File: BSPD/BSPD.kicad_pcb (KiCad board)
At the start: 2 copper layers, 1 part, among them J1 Conn_01x08

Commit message: finished V1 of bspd
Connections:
- J1 pad 1: unconnected-(J1-Pin_1-Pad1) -> +5V
- J1 pad 2: unconnected-(J1-Pin_2-Pad2) -> GND
- J1 pad 3: unconnected-(J1-Pin_3-Pad3) -> /Rear_Brake_Sensor
- J1 pad 4: unconnected-(J1-Pin_4-Pad4) -> /Front_Brake_Sensor
- J1 pad 5: unconnected-(J1-Pin_5-Pad5) -> /Current_Sensor_Output
- J1 pad 6: unconnected-(J1-Pin_6-Pad6) -> /Current_Sensor_VREF
- J1 pad 7: unconnected-(J1-Pin_7-Pad7) -> /Fault
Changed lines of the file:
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@@
 	)
 	(net 0 "")
-	(net 1 "unconnected-(J1-Pin_6-Pad6)")
+	(net 1 "/Current_Sensor_Output")
 	(net 2 "unconnected-(J1-Pin_8-Pad8)")
-	(net 3 "unconnected-(J1-Pin_3-Pad3)")
-	(net 4 "unconnected-(J1-Pin_4-Pad4)")
-	(net 5 "unconnected-(J1-Pin_7-Pad7)")
-	(net 6 "unconnected-(J1-Pin_2-Pad2)")
-	(net 7 "unconnected-(J1-Pin_1-Pad1)")
-	(net 8 "unconnected-(J1-Pin_5-Pad5)")
+	(net 3 "GND")
+	(net 4 "/Front_Brake_Sensor")
+	(net 5 "/Rear_Brake_Sensor")
+	(net 6 "+5V")
+	(net 7 "/Current_Sensor_VREF")
+	(net 8 "/Fault")
 	(footprint "Connector_Molex:Molex_Nano-Fit_105313-xx08_1x08_P2.50mm_Horizontal"
 		(layer "F.Cu")
@@
 			(remove_unused_layers no)
 			(roundrect_rratio 0.147059)
-			(net 7 "unconnected-(J1-Pin_1-Pad1)")
+			(net 6 "+5V")
 			(pinfunction "Pin_1")
 			(pintype "passive")
@@
 			(layers "*.Cu" "*.Mask")
 			(remove_unused_layers no)
-			(net 6 "unconnected-(J1-Pin_2-Pad2)")
+			(net 3 "GND")
 			(pinfunction "Pin_2")
 			(pintype "passive")
@@
 			(layers "*.Cu" "*.Mask")
 			(remove_unused_layers no)
-			(net 3 "unconnected-(J1-Pin_3-Pad3)")
+			(net 5 "/Rear_Brake_Sensor")
 			(pinfunction "Pin_3")
 			(pintype "passive")
@@
 			(layers "*.Cu" "*.Mask")
 			(remove_unused_layers no)
-			(net 4 "unconnected-(J1-Pin_4-Pad4)")
+			(net 4 "/Front_Brake_Sensor")
 			(pinfunction "Pin_4")
 			(pintype "passive")
@@
 			(layers "*.Cu" "*.Mask")
 			(remove_unused_layers no)
-			(net 8 "unconnected-(J1-Pin_5-Pad5)")
+			(net 1 "/Current_Sensor_Output")
 			(pinfunction "Pin_5")
 			(pintype "passive")
@@
 			(layers "*.Cu" "*.Mask")
 			(remove_unused_layers no)
-			(net 1 "unconnected-(J1-Pin_6-Pad6)")
+			(net 7 "/Current_Sensor_VREF")
 			(pinfunction "Pin_6")
 			(pintype "passive")
@@
 			(layers "*.Cu" "*.Mask")
 			(remove_unused_layers no)
-			(net 5 "unconnected-(J1-Pin_7-Pad7)")
+			(net 8 "/Fault")
 			(pinfunction "Pin_7")
 			(pintype "passive")

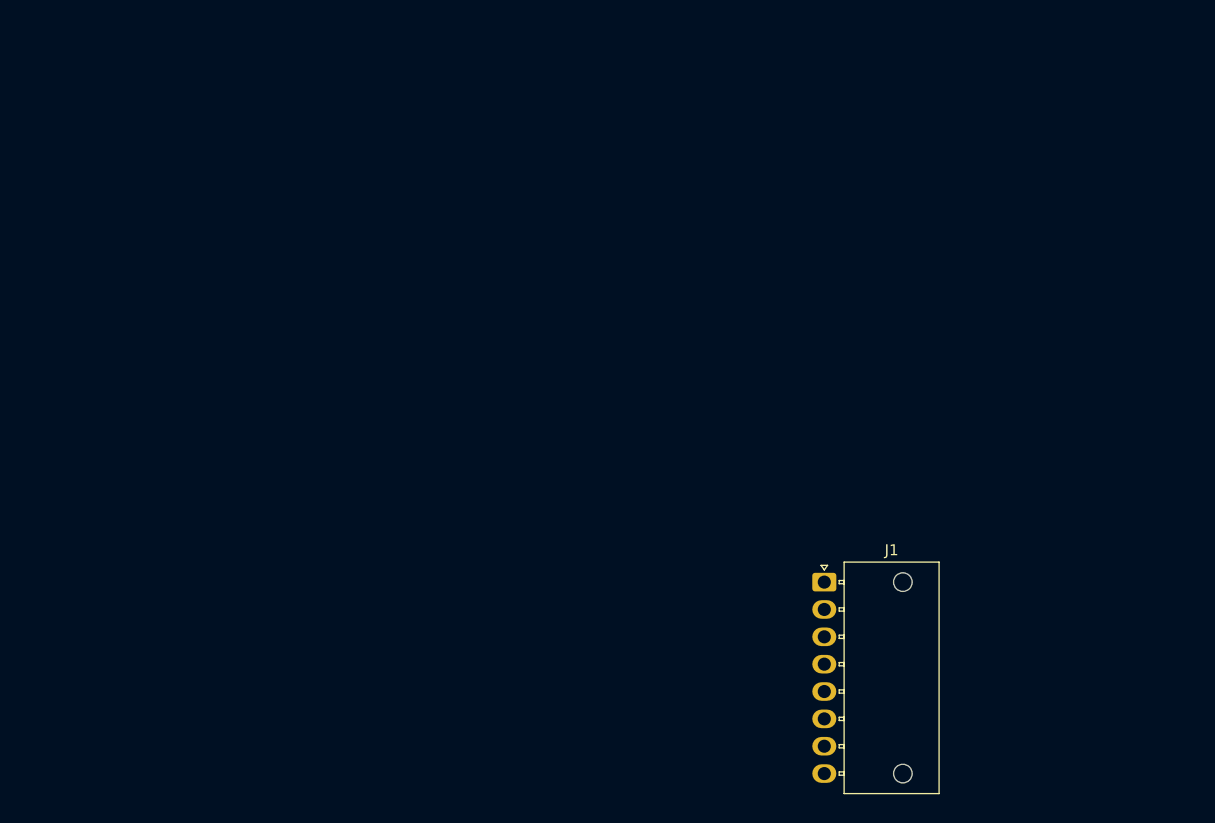
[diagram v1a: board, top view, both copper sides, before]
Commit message: Finished BSPD
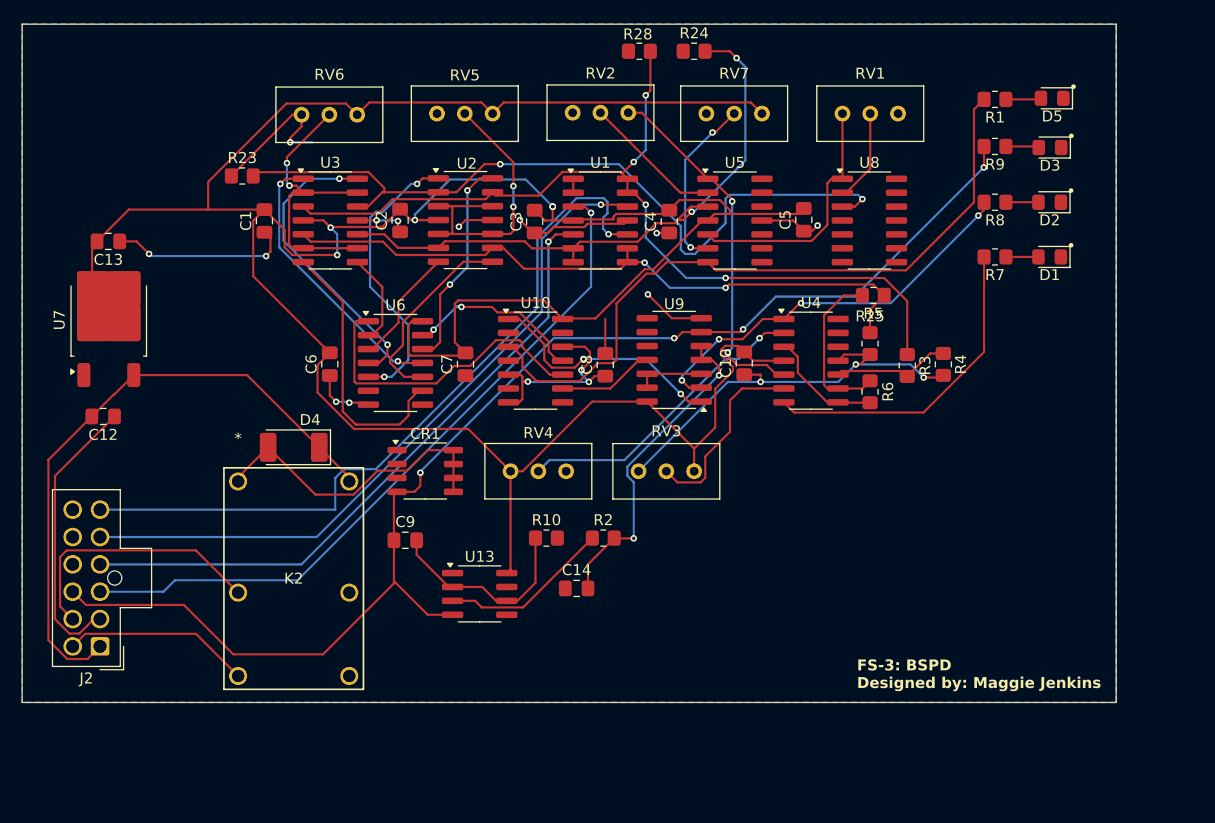
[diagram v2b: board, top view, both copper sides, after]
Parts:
- removed J1: Conn_01x08, Connector_Molex:Molex_Nano-Fit_105313-xx08_1x08_P2.50mm_Horizontal
- added C1: 0.1μF, Capacitor_SMD:C_0805_2012Metric_Pad1.18x1.45mm_HandSolder, F.Cu at (35.1, 33.0)
- added C10: 0.1μF, Capacitor_SMD:C_0805_2012Metric_Pad1.18x1.45mm_HandSolder, F.Cu at (79.0, 46.0)
- added C12: 0.33µF, Capacitor_SMD:C_0805_2012Metric_Pad1.18x1.45mm_HandSolder, F.Cu at (20.4, 50.9)
- added C13: 0.1µF, Capacitor_SMD:C_0805_2012Metric_Pad1.18x1.45mm_HandSolder, F.Cu at (20.9, 34.9)
- added C14: 0.1μF, Capacitor_SMD:C_0805_2012Metric_Pad1.18x1.45mm_HandSolder, F.Cu at (63.7, 66.6)
- added C2: 0.1μF, Capacitor_SMD:C_0805_2012Metric_Pad1.18x1.45mm_HandSolder, F.Cu at (47.5, 32.9)
- added C3: 0.1μF, Capacitor_SMD:C_0805_2012Metric_Pad1.18x1.45mm_HandSolder, F.Cu at (59.8, 33.0)
- added C4: 0.1μF, Capacitor_SMD:C_0805_2012Metric_Pad1.18x1.45mm_HandSolder, F.Cu at (72.1, 33.0)
- added C5: 0.1μF, Capacitor_SMD:C_0805_2012Metric_Pad1.18x1.45mm_HandSolder, F.Cu at (84.4, 32.9)
- added C6: 0.1μF, Capacitor_SMD:C_0805_2012Metric_Pad1.18x1.45mm_HandSolder, F.Cu at (41.1, 46.1)
- added C7: 0.1μF, Capacitor_SMD:C_0805_2012Metric_Pad1.18x1.45mm_HandSolder, F.Cu at (53.5, 46.1)
- added C8: 0.1μF, Capacitor_SMD:C_0805_2012Metric_Pad1.18x1.45mm_HandSolder, F.Cu at (66.3, 46.1)
- added C9: 1µF, Capacitor_SMD:C_0805_2012Metric_Pad1.18x1.45mm_HandSolder, F.Cu at (48.0, 62.2)
- added CR1: STS6NF20V, Package_SO:SO-8_3.9x4.9mm_P1.27mm, F.Cu at (49.8, 55.8)
- added D1: QBLP631-R3A, FS_3_Global_Footprint_Library:LED_0805_2012Metric_Pad1.15x1.40mm_HandSolder_CathodeDot, F.Cu at (106.9, 36.3)
- added D2: QBLP631-R3A, FS_3_Global_Footprint_Library:LED_0805_2012Metric_Pad1.15x1.40mm_HandSolder_CathodeDot, F.Cu at (106.9, 31.3)
- added D3: QBLP631-R3A, FS_3_Global_Footprint_Library:LED_0805_2012Metric_Pad1.15x1.40mm_HandSolder_CathodeDot, F.Cu at (106.9, 26.3)
- added D4: D, Diode_SMD:D_2010_5025Metric_Pad1.52x2.65mm_HandSolder, F.Cu at (37.8, 53.7)
- added D5: QBLP631-R3A, FS_3_Global_Footprint_Library:LED_0805_2012Metric_Pad1.15x1.40mm_HandSolder_CathodeDot, F.Cu at (107.1, 21.8)
- added J2: Conn_01x12, Connector_Molex:Molex_Nano-Fit_105310-xx12_2x06_P2.50mm_Vertical, F.Cu at (20.1, 71.9)
- added K2: DK1A1B-12V, FS_3_Global_Footprint_Library:DK1A1B, F.Cu at (32.7, 56.8)
- added R1: 300, Resistor_SMD:R_0805_2012Metric_Pad1.20x1.40mm_HandSolder, F.Cu at (101.9, 21.9)
- added R10: 430k, Resistor_SMD:R_0805_2012Metric_Pad1.20x1.40mm_HandSolder, F.Cu at (60.9, 62.0)
- added R2: 10k, Resistor_SMD:R_0805_2012Metric_Pad1.20x1.40mm_HandSolder, F.Cu at (66.1, 62.0)
- added R23: 100k, Resistor_SMD:R_0805_2012Metric_Pad1.20x1.40mm_HandSolder, F.Cu at (33.1, 28.9)
- added R24: 100k, Resistor_SMD:R_0805_2012Metric_Pad1.20x1.40mm_HandSolder, F.Cu at (74.4, 17.5)
- added R25: 100k, Resistor_SMD:R_0805_2012Metric_Pad1.20x1.40mm_HandSolder, F.Cu at (90.5, 44.2)
- added R28: 100k, Resistor_SMD:R_0805_2012Metric_Pad1.20x1.40mm_HandSolder, F.Cu at (69.4, 17.5)
- added R3: 1k, Resistor_SMD:R_0805_2012Metric_Pad1.20x1.40mm_HandSolder, F.Cu at (93.9, 46.2)
- added R4: 20k, Resistor_SMD:R_0805_2012Metric_Pad1.20x1.40mm_HandSolder, F.Cu at (97.2, 46.1)
- added R5: 1k, Resistor_SMD:R_0805_2012Metric_Pad1.20x1.40mm_HandSolder, F.Cu at (90.8, 39.8)
- added R6: 20k, Resistor_SMD:R_0805_2012Metric_Pad1.20x1.40mm_HandSolder, F.Cu at (90.5, 48.6)
- added R7: 300, Resistor_SMD:R_0805_2012Metric_Pad1.20x1.40mm_HandSolder, F.Cu at (101.9, 36.3)
- added R8: 300, Resistor_SMD:R_0805_2012Metric_Pad1.20x1.40mm_HandSolder, F.Cu at (101.9, 31.3)
- added R9: 300, Resistor_SMD:R_0805_2012Metric_Pad1.20x1.40mm_HandSolder, F.Cu at (101.9, 26.2)
- added RV1: 3296W_10K, Potentiometer_THT:Potentiometer_Bourns_3296W_Vertical, F.Cu at (93.1, 23.2)
- added RV2: 3296W_10K, Potentiometer_THT:Potentiometer_Bourns_3296W_Vertical, F.Cu at (63.3, 23.1)
- added RV3: 3296W_10K, Potentiometer_THT:Potentiometer_Bourns_3296W_Vertical, F.Cu at (74.4, 55.9)
- added RV4: 3296W_10K, Potentiometer_THT:Potentiometer_Bourns_3296W_Vertical, F.Cu at (57.6, 55.9)
- added RV5: 3296W_10K, Potentiometer_THT:Potentiometer_Bourns_3296W_Vertical, F.Cu at (56.0, 23.2)
- added RV6: 3296W_10K, Potentiometer_THT:Potentiometer_Bourns_3296W_Vertical, F.Cu at (43.6, 23.3)
- added RV7: 3296W_10K, Potentiometer_THT:Potentiometer_Bourns_3296W_Vertical, F.Cu at (80.6, 23.2)
- added U1: MCP6004, Package_SO:SOIC-14_3.9x8.7mm_P1.27mm, F.Cu at (65.8, 32.9)
- added U10: 4072, Package_SO:SOIC-14_3.9x8.7mm_P1.27mm, F.Cu at (59.9, 45.8)
- added U13: LM555xM, Package_SO:SOIC-8_3.9x4.9mm_P1.27mm, F.Cu at (54.8, 67.1)
- added U2: MCP6004, Package_SO:SOIC-14_3.9x8.7mm_P1.27mm, F.Cu at (53.5, 32.9)
- added U3: MCP6004, Package_SO:SOIC-14_3.9x8.7mm_P1.27mm, F.Cu at (41.2, 32.9)
- added U4: MCP6004, Package_SO:SOIC-14_3.9x8.7mm_P1.27mm, F.Cu at (85.1, 45.8)
- added U5: MCP6004, Package_SO:SOIC-14_3.9x8.7mm_P1.27mm, F.Cu at (78.1, 32.9)
- added U6: 4072, Package_SO:SOIC-14_3.9x8.7mm_P1.27mm, F.Cu at (47.1, 46.0)
- added U7: LD1086DT50TR, Package_TO_SOT_SMD:TO-252-2, F.Cu at (20.9, 42.0)
- added U8: MCP6004, Package_SO:SOIC-14_3.9x8.7mm_P1.27mm, F.Cu at (90.4, 32.9)
- added U9: 74HC00, Package_SO:SOIC-14_3.9x8.7mm_P1.27mm, F.Cu at (72.6, 45.7)
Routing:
- net +5V: track 0.00 -> 290.0 mm, vias 0 -> 5
- net GND: track 0.00 -> 151.6 mm, vias 0 -> 18
- net /BSPD_Fault_LOW: track 0.00 -> 118.1 mm, vias 0 -> 4
- net /Current_Sensor_Output_Buffered: track 0.00 -> 81.9 mm, vias 0 -> 4
- net /Rear_Brake_Buffered: track 0.00 -> 71.7 mm, vias 0 -> 2
- net /Current_Sensor_VREF: track 0.00 -> 68.8 mm, vias 0 -> 1
- net /Rear_Brake_Sensor: track 0.00 -> 65.0 mm, vias 0 -> 1
- net /Current_Sensor_Output: track 0.00 -> 64.8 mm, vias 0 -> 1
- net /rear_hard_braking: track 0.00 -> 64.6 mm
- net /Current_Sensor_VREF_Buffered: track 0.00 -> 61.9 mm, vias 0 -> 2
- net /Front_Brake_Sensor: track 0.00 -> 59.8 mm, vias 0 -> 1
- net +12V: track 0.00 -> 57.6 mm
- net /Front_Brake_Buffered: track 0.00 -> 57.2 mm, vias 0 -> 2
- net /high_current: track 0.00 -> 37.0 mm, vias 0 -> 4
- net /differential_front_brake_output: track 0.00 -> 33.1 mm, vias 0 -> 2
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- added copper zone on B.Cu, net GND
- added copper zone on F.Cu, net GND
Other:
- board outline added: 100 x 62 mm
- board text added: "FS-3: BSPD Designed by: Maggie Jenkins"
- board text added: "U2"

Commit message: all BSPD changes
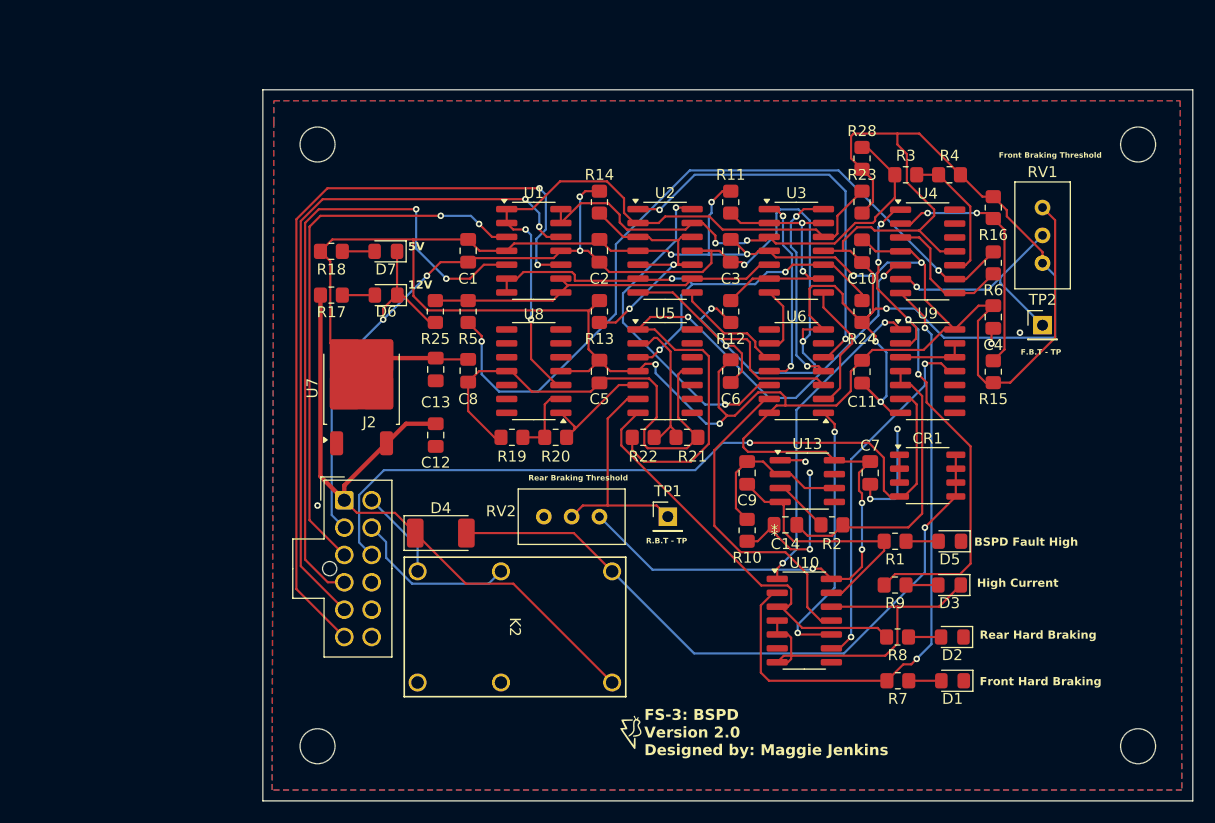
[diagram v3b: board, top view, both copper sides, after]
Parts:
- removed RV3, RV4, RV5, RV6, RV7: 3296W_10K, Potentiometer_THT:Potentiometer_Bourns_3296W_Vertical
- added C11: 0.1μF, Capacitor_SMD:C_0805_2012Metric_Pad1.18x1.45mm_HandSolder, F.Cu at (89.8, 46.8)
- added D6: QBLP631-R3A, LED_SMD:LED_0805_2012Metric_Pad1.15x1.40mm_HandSolder, F.Cu at (46.3, 39.8)
- added D7: QBLP631-R3A, LED_SMD:LED_0805_2012Metric_Pad1.15x1.40mm_HandSolder, F.Cu at (46.2, 35.8)
- added G***: LOGO, FS_3_Global_Footprint_Library:FORMULA SLUG, F.Cu at (71.8, 79.8)
- added R11: 3.9k, Resistor_SMD:R_0805_2012Metric_Pad1.20x1.40mm_HandSolder, F.Cu at (77.8, 31.3)
- added R12: 33k, Resistor_SMD:R_0805_2012Metric_Pad1.20x1.40mm_HandSolder, F.Cu at (77.8, 41.3)
- added R13: 22k, Resistor_SMD:R_0805_2012Metric_Pad1.20x1.40mm_HandSolder, F.Cu at (65.8, 41.3)
- added R14: 1.2k, Resistor_SMD:R_0805_2012Metric_Pad1.20x1.40mm_HandSolder, F.Cu at (65.8, 31.3)
- added R15: 12k, Resistor_SMD:R_0805_2012Metric_Pad1.20x1.40mm_HandSolder, F.Cu at (101.8, 46.8)
- added R16: 15k, Resistor_SMD:R_0805_2012Metric_Pad1.20x1.40mm_HandSolder, F.Cu at (101.8, 31.8)
- added R17: 1k, Resistor_SMD:R_0805_2012Metric_Pad1.20x1.40mm_HandSolder, F.Cu at (41.3, 39.8)
- added R18: 330, Resistor_SMD:R_0805_2012Metric_Pad1.20x1.40mm_HandSolder, F.Cu at (41.3, 35.8)
- added R19: 10k, Resistor_SMD:R_0805_2012Metric_Pad1.20x1.40mm_HandSolder, F.Cu at (57.8, 52.8)
- added R20: 10k, Resistor_SMD:R_0805_2012Metric_Pad1.20x1.40mm_HandSolder, F.Cu at (61.8, 52.8)
- added R21: 10k, Resistor_SMD:R_0805_2012Metric_Pad1.20x1.40mm_HandSolder, F.Cu at (73.8, 52.8)
- added R22: 10k, Resistor_SMD:R_0805_2012Metric_Pad1.20x1.40mm_HandSolder, F.Cu at (69.8, 52.8)
- added REF**: MountingHole_3.2mm_M3, MountingHole:MountingHole_3.2mm_M3, F.Cu at (115.0, 26.0)
- added REF**: MountingHole_3.2mm_M3, MountingHole:MountingHole_3.2mm_M3, F.Cu at (115.0, 81.0)
- added REF**: MountingHole_3.2mm_M3, MountingHole:MountingHole_3.2mm_M3, F.Cu at (40.0, 26.0)
- added REF**: MountingHole_3.2mm_M3, MountingHole:MountingHole_3.2mm_M3, F.Cu at (40.0, 81.0)
- added TP1: rear_braking_threshold, Connector_PinHeader_2.54mm:PinHeader_1x01_P2.54mm_Vertical, F.Cu at (72.0, 60.0)
- added TP2: front_braking_threshold, Connector_PinHeader_2.54mm:PinHeader_1x01_P2.54mm_Vertical, F.Cu at (106.3, 42.5)
- D1, D2, D3, D5: footprint FS_3_Global_Footprint_Library:LED_0805_2012Metric_Pad1.15x1.40mm_HandSolder_CathodeDot -> LED_SMD:LED_0805_2012Metric_Pad1.15x1.40mm_HandSolder
- R1, R7, R8, R9: value 300 -> 330
- moved R23 56.7 mm to (89.8, 31.3), turned to 90 degrees
- moved CR1 45.9 mm to (95.8, 56.3)
- moved U3 42.7 mm to (83.8, 35.7)
- moved D5 41.6 mm to (97.8, 62.3)
- moved R1 41.4 mm to (92.8, 62.3)
- moved R9 41.1 mm to (92.8, 66.3)
- moved D3 41.0 mm to (97.8, 66.3)
- moved D2 40.7 mm to (98.0, 71.0)
- moved R8 40.7 mm to (93.0, 71.0)
- moved R25 39.8 mm to (50.8, 41.3)
- moved D1 39.7 mm to (98.0, 75.0)
- moved R7 39.7 mm to (93.0, 75.0)
- moved C7 38.3 mm to (90.5, 56.0)
- moved R5 37.1 mm to (53.8, 41.3), turned to -90 degrees
- moved RV2 37.0 mm to (65.8, 60.0), turned to 0 degrees
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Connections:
- C9 pad 1: /BSPD_Fault_LOW -> /BSPD_Fault_HIGH
- R1 pad 2: /rear_hard_braking -> /BSPD_Fault_HIGH
- R8 pad 2: /high_current -> /rear_hard_braking
- R9 pad 2: /BSPD_Fault_LOW -> /high_current
- RV1 pad 1: GND -> +5V
- RV1 pad 2: Net-(U8A--) -> /front_braking_threshhold
- RV1 pad 3: /differential_rear_brake_output -> GND
- RV2 pad 1: GND -> +5V
- RV2 pad 2: Net-(U5A--) -> /rear_braking_threshhold
- RV2 pad 3: /differential_front_brake_output -> GND
- U10 pad 2: /front_high_braking -> /front_hard_braking
- U13 pad 4: /BSPD_Fault_LOW -> /BSPD_Fault_HIGH
- U4 pad 5: /differential_front_brake_output -> /non_inv_front_brake_output
- U5 pad 1: /differential_front_brake_output -> /non_inv_front_brake_output
- U5 pad 5: /differential_rear_brake_output -> /non_inv_rear_brake_output
- U8 pad 1: /differential_rear_brake_output -> /non_inv_rear_brake_output
- U8 pad 11: (no net) -> GND
- U8 pad 4: (no net) -> +5V
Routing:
- net GND: track 151.6 -> 357.7 mm, vias 18 -> 19
- net /non_inv_front_brake_output: track 0.00 -> 59.2 mm, vias 0 -> 2
- net Net-(U4C--): track 15.3 -> 69.9 mm, vias 0 -> 2
- net /BSPD_Fault_LOW: track 118.1 -> 72.1 mm, vias 4 -> 1
- net /Current_Sensor_Output_Buffered: track 81.9 -> 44.0 mm, vias 4 -> 2
- net /differential_front_brake_output: track 33.1 -> 0.00 mm, vias 2 -> 0
- net Net-(D4-A): track 28.5 -> 61.5 mm, vias 0 -> 1
- net /Current_Sensor_VREF_Buffered: track 61.9 -> 32.8 mm, vias 2 -> 0
- net /front_hard_braking: track 29.7 -> 58.7 mm, vias 0 -> 2
- net /rear_hard_braking: track 64.6 -> 38.4 mm
- net /logic/hard_braking_high_current: track 8.81 -> 33.0 mm, vias 0 -> 2
- net /BSPD_Fault_HIGH: track 0.00 -> 23.4 mm
- net /differential_rear_brake_output: track 23.1 -> 0.00 mm
- net /current_VREF_short: track 25.0 -> 6.28 mm
- net +5V: track 290.0 -> 273.5 mm, vias 5 -> 10
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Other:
- board size 100 x 62 mm -> 85 x 65 mm
- board text added: "12V"
- board text added: "5V"
- board text added: "BSPD Fault High"
- board text added: "F.B.T - TP"
- board text added: "FS-3: BSPD Version 2.0 Designed by: Maggie Jenkins"
- board text added: "Front Braking Threshold"
- board text added: "Front Hard Braking"
- board text added: "High Current"
- board text added: "R.B.T - TP"
- board text added: "Rear Braking Threshold"
- board text added: "Rear Hard Braking"
- board text removed: "FS-3: BSPD Designed by: Maggie Jenkins"
- board text removed: "U2"
